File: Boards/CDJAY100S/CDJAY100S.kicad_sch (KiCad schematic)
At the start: 50 parts, among them SW1 RotaryEncoder_Switch, U1 HT1632C-52LQFP

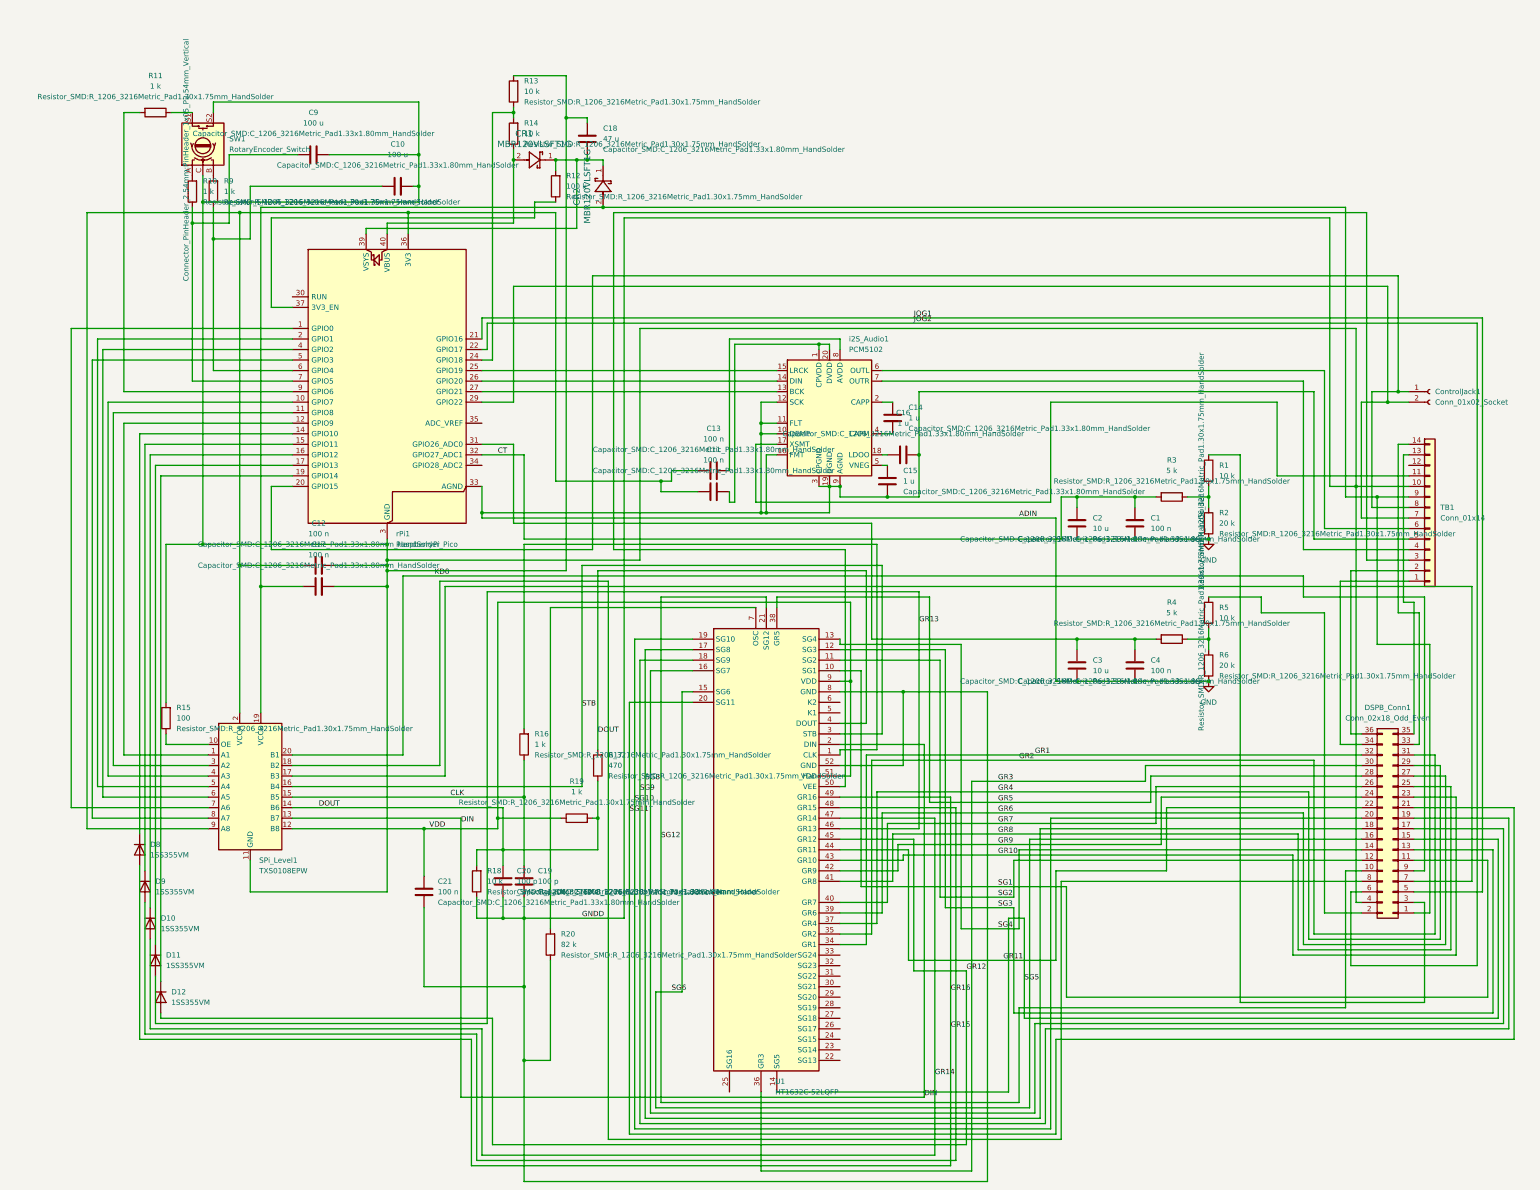
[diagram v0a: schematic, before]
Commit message: Hide some details
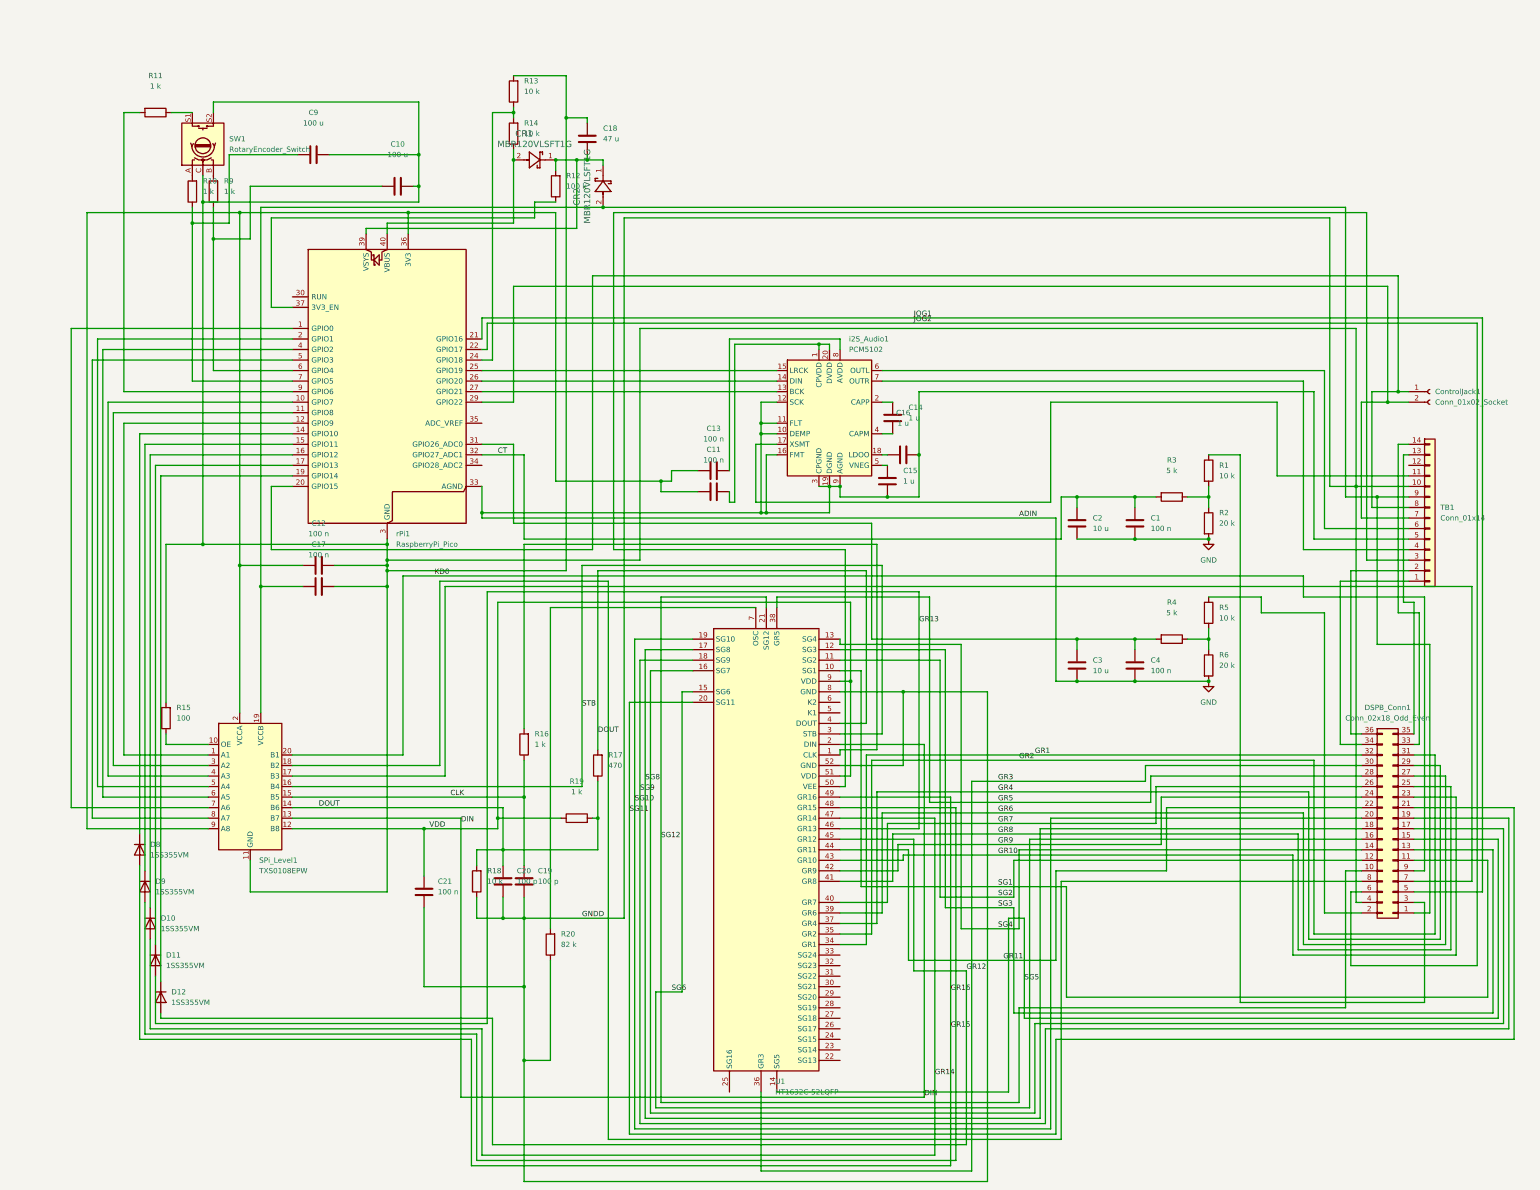
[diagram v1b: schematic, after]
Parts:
- C11: footprint Capacitor_SMD:C_1206_3216Metric_Pad1.33x1.80mm_HandSolder -> (none)
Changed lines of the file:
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@@
 		(property "Footprint" "Resistor_SMD:R_1206_3216Metric_Pad1.30x1.75mm_HandSolder"
 			(at 325.882 146.05 90)
+			(hide yes)
 			(show_name no)
 			(do_not_autoplace no)
@@
 		(property "Footprint" "Connector_PinHeader_2.54mm:PinHeader_1x05_P2.54mm_Vertical"
 			(at 81.026 36.83 0)
+			(hide yes)
 			(show_name no)
 			(do_not_autoplace no)
@@
 		(property "Footprint" "Resistor_SMD:R_1206_3216Metric_Pad1.30x1.75mm_HandSolder"
 			(at 171.45 228.5999 0)
+			(hide yes)
 			(show_name no)
 			(do_not_autoplace no)
@@
 		(property "Footprint" "Capacitor_SMD:C_1206_3216Metric_Pad1.33x1.80mm_HandSolder"
 			(at 111.76 30.48 90)
+			(hide yes)
 			(show_name no)
 			(do_not_autoplace no)
@@
 		(property "Footprint" "Capacitor_SMD:C_1206_3216Metric_Pad1.33x1.80mm_HandSolder"
 			(at 254 116.8399 0)
+			(hide yes)
 			(show_name no)
 			(do_not_autoplace no)
@@
 		(property "Footprint" "Resistor_SMD:R_1206_3216Metric_Pad1.30x1.75mm_HandSolder"
 			(at 318.77 148.59 90)
+			(hide yes)
 			(show_name no)
 			(do_not_autoplace no)
@@
 		(property "Footprint" "Resistor_SMD:R_1206_3216Metric_Pad1.30x1.75mm_HandSolder"
 			(at 78.74 173.9899 0)
+			(hide yes)
 			(show_name no)
 			(do_not_autoplace no)
@@
 		(property "Footprint" "Resistor_SMD:R_1206_3216Metric_Pad1.30x1.75mm_HandSolder"
 			(at 182.88 185.4199 0)
+			(hide yes)
 			(show_name no)
 			(do_not_autoplace no)
@@
 		(property "Footprint" "Capacitor_SMD:C_1206_3216Metric_Pad1.33x1.80mm_HandSolder"
 			(at 113.03 134.62 90)
+			(hide yes)
 			(show_name no)
 			(do_not_autoplace no)
@@
 		(property "Footprint" "Capacitor_SMD:C_1206_3216Metric_Pad1.33x1.80mm_HandSolder"
 			(at 310.8452 162.56 0)
+			(hide yes)
 			(show_name no)
 			(do_not_autoplace no)
@@
 		(property "Footprint" "Resistor_SMD:R_1206_3216Metric_Pad1.30x1.75mm_HandSolder"
 			(at 90.17 46.9899 0)
+			(hide yes)
 			(show_name no)
 			(do_not_autoplace no)
@@
 		(property "Footprint" "Resistor_SMD:R_1206_3216Metric_Pad1.30x1.75mm_HandSolder"
 			(at 325.882 111.76 90)
+			(hide yes)
 			(show_name no)
 			(do_not_autoplace no)
@@
 		(property "Footprint" "Capacitor_SMD:C_1206_3216Metric_Pad1.33x1.80mm_HandSolder"
 			(at 132.08 38.1 90)
+			(hide yes)
 			(show_name no)
 			(do_not_autoplace no)
@@
 		(property "Footprint" "Capacitor_SMD:C_1206_3216Metric_Pad1.33x1.80mm_HandSolder"
 			(at 296.8752 128.27 0)
+			(hide yes)
 			(show_name no)
 			(do_not_autoplace no)
@@
 		(property "Footprint" "Resistor_SMD:R_1206_3216Metric_Pad1.30x1.75mm_HandSolder"
 			(at 73.66 21.59 90)
+			(hide yes)
 			(show_name no)
 			(do_not_autoplace no)
@@
 		(property "Footprint" "Capacitor_SMD:C_1206_3216Metric_Pad1.33x1.80mm_HandSolder"
 			(at 165.8903 213.3599 0)
+			(hide yes)
 			(show_name no)
 			(do_not_autoplace no)
@@
 		(property "Footprint" "Capacitor_SMD:C_1206_3216Metric_Pad1.33x1.80mm_HandSolder"
 			(at 160.8103 213.3599 0)
+			(hide yes)
 			(show_name no)
 			(do_not_autoplace no)
@@
 		(property "Footprint" "Capacitor_SMD:C_1206_3216Metric_Pad1.33x1.80mm_HandSolder"
 			(at 255.27 101.5999 0)
+			(hide yes)
 			(show_name no)
 			(do_not_autoplace no)
@@
 		(property "Footprint" "Resistor_SMD:R_1206_3216Metric_Pad1.30x1.75mm_HandSolder"
 			(at 165.1 180.3399 0)
+			(hide yes)
 			(show_name no)
 			(do_not_autoplace no)
@@
 		(property "Footprint" "Resistor_SMD:R_1206_3216Metric_Pad1.30x1.75mm_HandSolder"
 			(at 330.2 126.9999 0)
+			(hide yes)
 			(show_name no)
 			(do_not_autoplace no)
@@
 		(property "Footprint" "Resistor_SMD:R_1206_3216Metric_Pad1.30x1.75mm_HandSolder"
 			(at 85.09 46.9899 0)
+			(hide yes)
 			(show_name no)
 			(do_not_autoplace no)
@@
 		(property "Footprint" "Capacitor_SMD:C_1206_3216Metric_Pad1.33x1.80mm_HandSolder"
 			(at 181.61 34.2899 0)
+			(hide yes)
 			(show_name no)
 			(do_not_autoplace no)
@@
 		(property "Footprint" "Capacitor_SMD:C_1206_3216Metric_Pad1.33x1.80mm_HandSolder"
 			(at 296.8752 162.56 0)
+			(hide yes)
 			(show_name no)
 			(do_not_autoplace no)
@@
 			)
 		)
-		(property "Footprint" "Capacitor_SMD:C_1206_3216Metric_Pad1.33x1.80mm_HandSolder"
+		(property "Footprint" ""
 			(at 208.28 111.76 90)
-			(show_name no)
+			(hide yes)
+			(show_name yes)
 			(do_not_autoplace no)
 			(effects
 				(font
+					(face "KiCad Font")
 					(size 1.27 1.27)
 				)
@@
 		(property "Footprint" "Resistor_SMD:R_1206_3216Metric_Pad1.30x1.75mm_HandSolder"
 			(at 162.56 22.8599 0)
+			(hide yes)
 			(show_name no)
 			(do_not_autoplace no)
@@
 		(property "Footprint" "Resistor_SMD:R_1206_3216Metric_Pad1.30x1.75mm_HandSolder"
 			(at 318.77 114.3 90)
+			(hide yes)
 			(show_name no)
 			(do_not_autoplace no)
@@
 		(property "Footprint" "Capacitor_SMD:C_1206_3216Metric_Pad1.33x1.80mm_HandSolder"
 			(at 310.8452 128.27 0)
+			(hide yes)
 			(show_name no)
 			(do_not_autoplace no)
@@
 		(property "Footprint" "Resistor_SMD:R_1206_3216Metric_Pad1.30x1.75mm_HandSolder"
 			(at 162.56 33.0199 0)
+			(hide yes)
 			(show_name no)
 			(do_not_autoplace no)
@@
 		(property "Footprint" "Capacitor_SMD:C_1206_3216Metric_Pad1.33x1.80mm_HandSolder"
 			(at 113.03 129.54 90)
+			(hide yes)
 			(show_name no)
 			(do_not_autoplace no)
@@
 		(property "Footprint" "Resistor_SMD:R_1206_3216Metric_Pad1.30x1.75mm_HandSolder"
 			(at 330.2 161.2899 0)
+			(hide yes)
 			(show_name no)
 			(do_not_autoplace no)
@@
 		(property "Footprint" "Resistor_SMD:R_1206_3216Metric_Pad1.30x1.75mm_HandSolder"
 			(at 175.26 191.77 90)
+			(hide yes)
 			(show_name no)
 			(do_not_autoplace no)
@@
 		(property "Footprint" "Resistor_SMD:R_1206_3216Metric_Pad1.30x1.75mm_HandSolder"
 			(at 172.72 45.7199 0)
+			(hide yes)
 			(show_name no)
 			(do_not_autoplace no)
@@
 		(property "Footprint" "Capacitor_SMD:C_1206_3216Metric_Pad1.33x1.80mm_HandSolder"
 			(at 208.28 106.68 90)
+			(hide yes)
 			(show_name no)
 			(do_not_autoplace no)
@@
 		(property "Footprint" "Capacitor_SMD:C_1206_3216Metric_Pad1.33x1.80mm_HandSolder"
 			(at 254 102.87 90)
+			(hide yes)
 			(show_name no)
 			(do_not_autoplace no)
@@
 		(property "Footprint" "Capacitor_SMD:C_1206_3216Metric_Pad1.33x1.80mm_HandSolder"
 			(at 141.7603 215.8999 0)
+			(hide yes)
 			(show_name no)
 			(do_not_autoplace no)
@@
 		(property "Footprint" "Resistor_SMD:R_1206_3216Metric_Pad1.30x1.75mm_HandSolder"
 			(at 153.67 213.3599 0)
+			(hide yes)
 			(show_name no)
 			(do_not_autoplace no)
